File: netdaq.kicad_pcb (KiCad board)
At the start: 2 copper layers, 131.5 x 93 mm, 289 parts, among them J1 RJ45, J3 Conn_01x06_Pin, J4 Micro_SD_Card_Det2, U1 PIC32CK1025GC01100-I/4SB, U10 TLA2518IRTER, U11 TLA2518IRTER, U2 LAN8720A-CP, U5 MP6004GQ-P, U6 PD70100ILD-TR, U7 TPS62A01PDDCR, U8 TLA2518IRTER, U9 TLA2518IRTER, Y4 Crystal_GND24

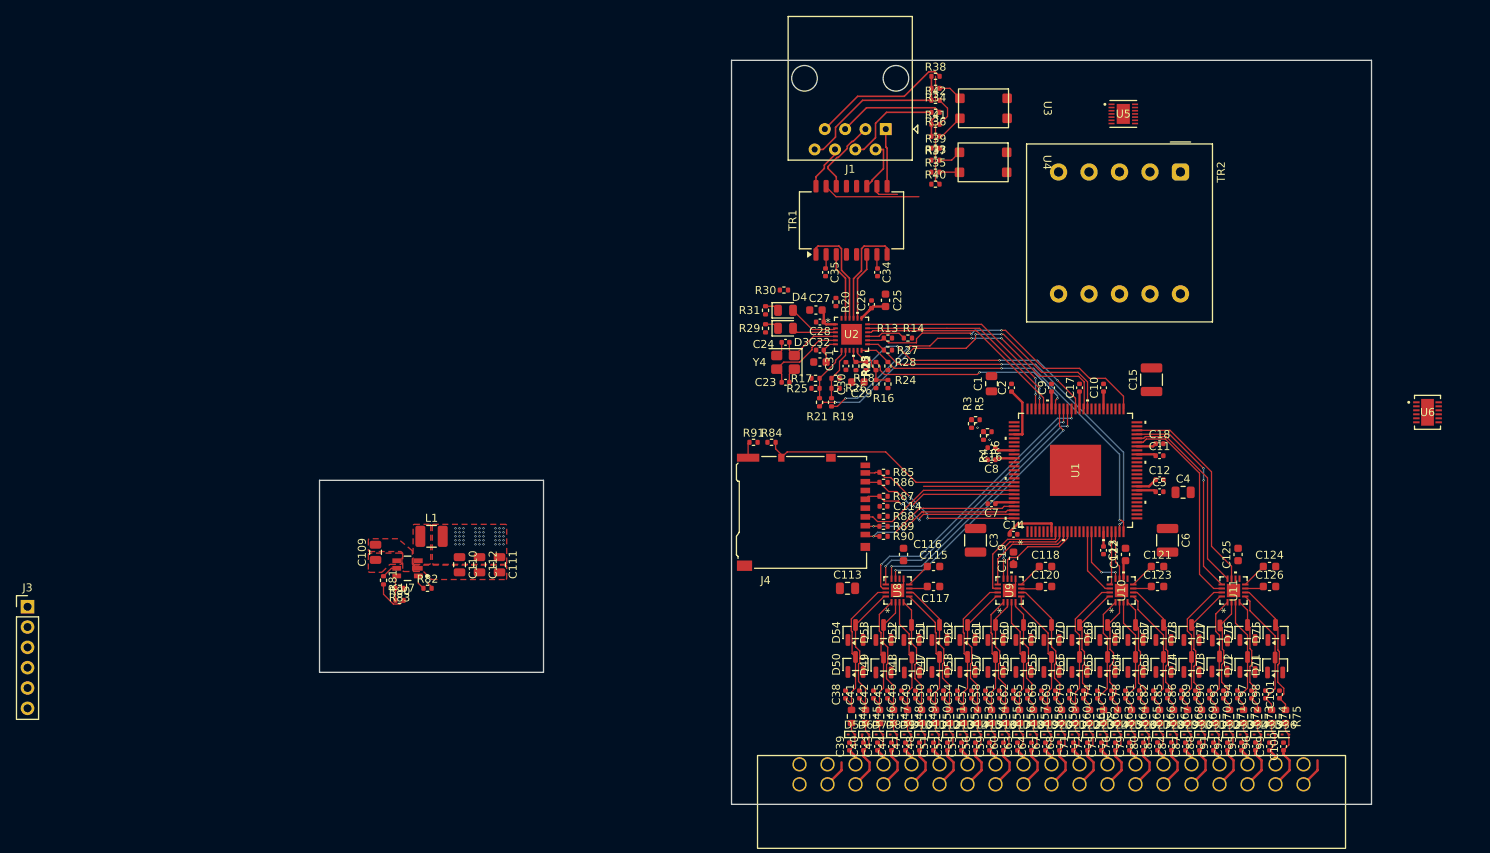
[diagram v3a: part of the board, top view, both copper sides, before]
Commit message: lots
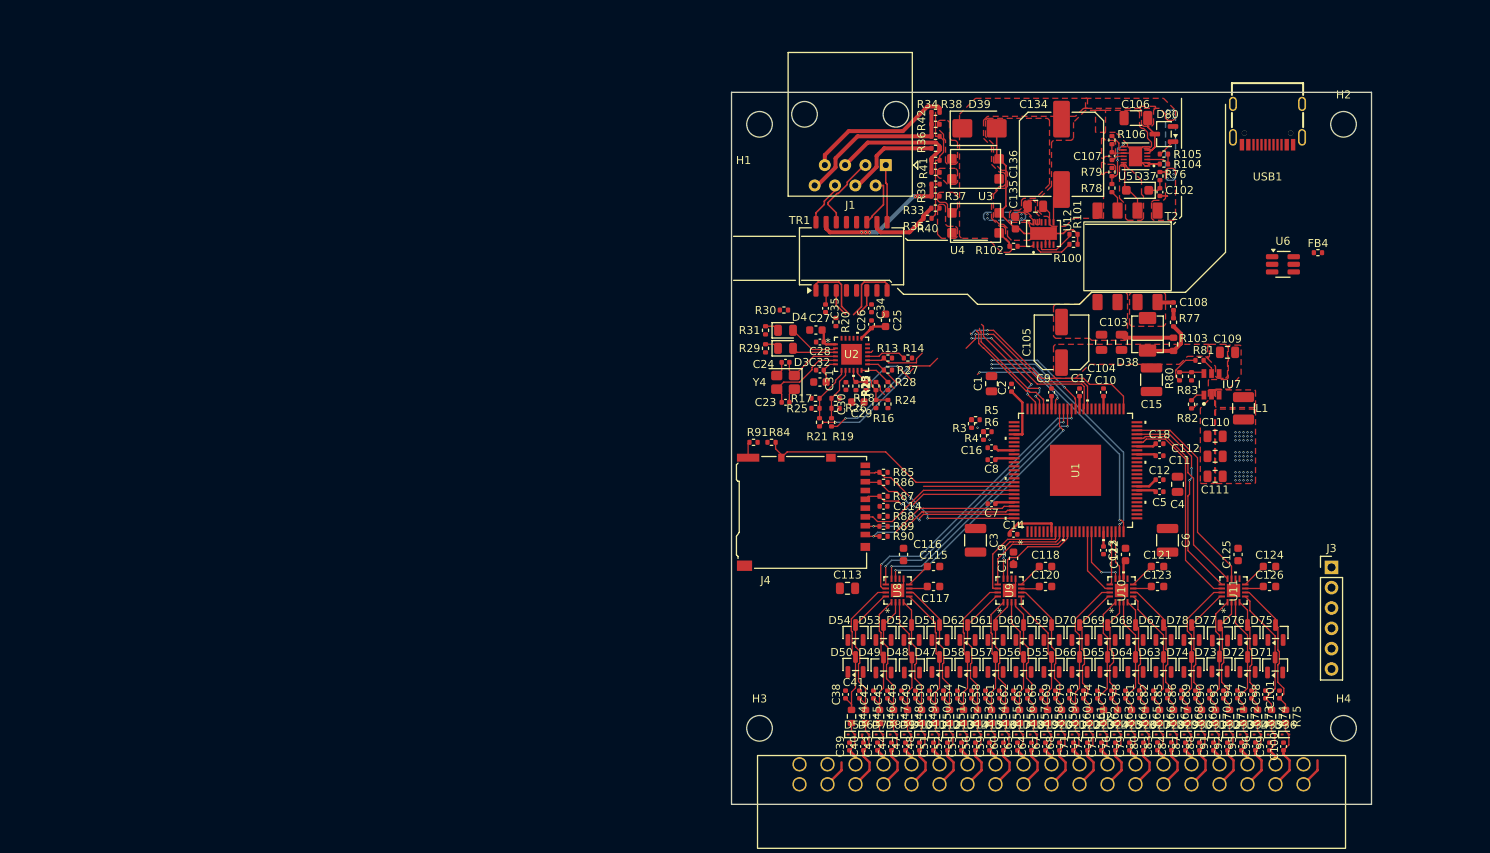
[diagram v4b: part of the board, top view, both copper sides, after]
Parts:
- removed TR2: Wuerth_750343373, Transformer_THT:Transformer_Wuerth_750343373
- added C102: 910p, Capacitor_SMD:C_0402_1005Metric, F.Cu at (183.6, 68.5)
- added C103: 22u 10 V, Capacitor_SMD:C_0805_2012Metric, F.Cu at (178.8, 87.2)
- added C104: 22u 10 V, Capacitor_SMD:C_0805_2012Metric, F.Cu at (176.2, 87.2)
- added C105: 220u, Capacitor_SMD:C_Elec_6.3x7.7, F.Cu at (171.2, 87.2)
- added C106: 2.2u 100 V, Capacitor_SMD:C_1206_3216Metric, F.Cu at (180.6, 59.2)
- added C107: 1u 10V, Capacitor_SMD:C_0402_1005Metric, F.Cu at (177.6, 64.0)
- added C108: C, Capacitor_SMD:C_0402_1005Metric, F.Cu at (185.2, 82.8)
- added C134: 47u, Capacitor_SMD:C_Elec_10x10.2, F.Cu at (171.2, 63.8)
- added C135: 100n 100V, Capacitor_SMD:C_0603_1608Metric, F.Cu at (165.5, 72.3)
- added C136: 4.7u, Capacitor_SMD:C_0805_2012Metric, F.Cu at (168.0, 70.2)
- added D37: US1MFA, Diode_SMD:D_SOD-123F, F.Cu at (180.8, 68.2)
- added D38: VS-10BQ060-M3/5BT, SMB:SMB(DO-214AA), F.Cu at (182.0, 86.2)
- added D39: SMBJ58A, Diode_SMD:D_SMB, F.Cu at (161.0, 60.5)
- added D80: MMBZ5256ELT1G, MMBZ5256ELT1G:SOT-23(1-3), F.Cu at (184.1, 61.2)
- added FB4: FerriteBead, Resistor_SMD:R_0402_1005Metric, F.Cu at (203.3, 76.0)
- added H1: MountingHole, MountingHole:MountingHole_3.2mm_M3_ISO14580, F.Cu at (133.5, 60.0)
- added H2: MountingHole, MountingHole:MountingHole_3.2mm_M3_ISO14580, F.Cu at (206.5, 60.0)
- added H3: MountingHole, MountingHole:MountingHole_3.2mm_M3_ISO14580, F.Cu at (133.5, 135.5)
- added H4: MountingHole, MountingHole:MountingHole_3.2mm_M3_ISO14580, F.Cu at (206.5, 135.5)
- added R100: 240k, Resistor_SMD:R_0402_1005Metric, F.Cu at (172.8, 75.0)
- added R101: 133, Resistor_SMD:R_0402_1005Metric, F.Cu at (172.8, 73.8)
- added R102: 24.9k, Resistor_SMD:R_0402_1005Metric, F.Cu at (165.2, 75.2)
- added R103: 500, Resistor_SMD:R_0603_1608Metric, F.Cu at (185.2, 87.5)
- added R104: 13k, Resistor_SMD:R_0402_1005Metric, F.Cu at (184.1, 65.0)
- added R105: 10k, Resistor_SMD:R_0402_1005Metric, F.Cu at (184.1, 63.7)
- added R106: 330k, Resistor_SMD:R_0402_1005Metric, F.Cu at (177.6, 62.0)
- added R76: 56k, Resistor_SMD:R_0402_1005Metric, F.Cu at (183.6, 66.5)
- added R77: R, Resistor_SMD:R_0402_1005Metric, F.Cu at (185.2, 84.8)
- added R78: 68k, Resistor_SMD:R_0402_1005Metric, F.Cu at (177.6, 68.0)
- added R79: 12k, Resistor_SMD:R_0402_1005Metric, F.Cu at (177.6, 66.0)
- added T2: POE30P-50L, POE30P-50L:POE30P-50L, F.Cu at (179.5, 76.5)
- added U12: PD70100ILD-TR, PD70100ILD-TR:DFN12_4X3_MCH, F.Cu at (169.0, 73.6)
- added USB1: HYCW498-USBC16-735B, C42400252:USB-C-SMD_HYCW498-USBC16-735B, F.Cu at (197.0, 60.0)
- U6: value PD70100ILD-TR -> TPUSBLC6-4SC6; footprint PD70100ILD-TR:DFN12_4X3_MCH -> Package_TO_SOT_SMD:SOT-23-6_Handsoldering
- moved J3 163.1 mm to (205.0, 115.4)
- moved C109 109.4 mm to (192.0, 88.5), turned to 0 degrees
- moved R81 105.6 mm to (188.5, 89.5), turned to 180 degrees
- moved U7 103.1 mm to (190.0, 92.5), turned to 90 degrees
- moved L1 102.8 mm to (194.0, 95.5), turned to -90 degrees
- moved R83 102.5 mm to (187.5, 91.5), turned to 90 degrees
- moved R80 101.4 mm to (186.0, 91.5), turned to -90 degrees
- moved R82 98.2 mm to (187.5, 95.0), turned to -90 degrees
- moved C110 95.8 mm to (190.4, 99.0), turned to 180 degrees
- moved C112 92.9 mm to (190.4, 101.5), turned to 180 degrees
- moved C111 90.1 mm to (190.4, 104.0), turned to 180 degrees
- moved U6 25.9 mm to (198.9, 77.5)
- moved U3 7.64 mm to (160.5, 65.6)
- moved U4 7.63 mm to (160.5, 72.3)
- moved U5 5.52 mm to (180.5, 64.0), turned to 180 degrees
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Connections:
- U5 pad 1: ETH_SHIELD -> PGND
- U5 pad 10: ETH_SHIELD -> PGND
- U5 pad 15: ETH_SHIELD -> PGND
- U5 pad 2: ETH_SHIELD -> PGND
- U5 pad 3: unconnected-(U5-EN-Pad3) -> /PoE Regulator/FLY_EN
- U5 pad 5: /PoE Regulator/VIN -> /Ethernet Connector/POE_V+
- U5 pad 6: /PoE Regulator/VIN -> /Ethernet Connector/POE_V+
- U5 pad 7: unconnected-(U5-MODE-Pad7) -> PGND
- U5 pad 9: unconnected-(U5-ILIM-Pad9) -> Net-(U5-ILIM)
- U6 pad 1: unconnected-(U6-RDET-Pad1) -> /USB.D+
- U6 pad 2: unconnected-(U6-RREF-Pad2) -> GND
- U6 pad 5: unconnected-(U6-VPNIN-Pad5) -> /USB Connector/EXT_VBUS
- U6 pad 6: unconnected-(U6-NC-Pad6) -> /USB.D-
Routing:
- net /Ethernet Connector/POE_V-: track 0.00 -> 27.2 mm
- net PGND: track 0.00 -> 20.2 mm
- net /RMII.TXD1: track 27.6 -> 13.8 mm
- net /RMII.TXD0: track 27.2 -> 14.5 mm
- net /SMI.MDIO: track 47.7 -> 35.5 mm
- net /RMII.TXEN: track 26.9 -> 14.8 mm
- net /SMI.MDC: track 47.8 -> 36.1 mm
- net /RMII.CRSDV: track 26.7 -> 15.1 mm
- net /Ethernet Connector/POE_V+: track 0.00 -> 10.5 mm, vias 0 -> 16
- net /RMII.RXER: track 34.3 -> 24.3 mm
- net +5.0V: track 0.91 -> 8.01 mm
- net /RMII.RXD1: track 43.4 -> 36.5 mm
- net /PoE Regulator/FLY_SW: track 0.00 -> 6.70 mm
- net GND: track 12.2 -> 18.8 mm
- net /PoE Regulator/FLY_FB: track 0.00 -> 6.29 mm, vias 0 -> 2
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- added copper zone on F.Cu, net /Ethernet Connector/POE_CT1
- added copper zone on F.Cu, net /Ethernet Connector/POE_CT2
- added copper zone on B.Cu, net /Ethernet Connector/POE_V+
- added copper zone on F.Cu, net /Ethernet Connector/POE_V+
- added copper zone on F.Cu, net /Ethernet Connector/POE_V-
- added copper zone on F.Cu, net /PD Controller/PD_AUX
- added copper zone on F.Cu, net /PoE Regulator/FLY_SW
- added copper zone on F.Cu, net Net-(D38-A)
- added copper zone on F.Cu, net Net-(R33-Pad1)
- added copper zone on F.Cu, net Net-(R34-Pad1)
- added copper zone on F.Cu, net PGND
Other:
- board size 131.5 x 93 mm -> 80 x 89 mm
- board text removed: "3v3"
